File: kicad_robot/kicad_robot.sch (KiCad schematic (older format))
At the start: 1 part

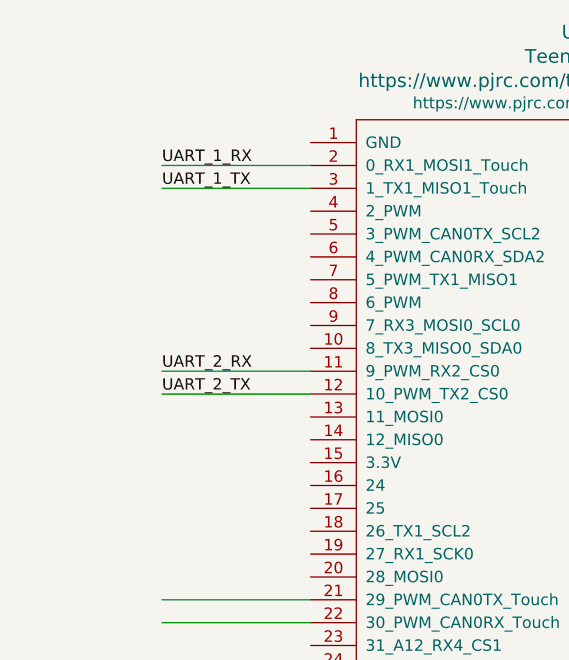
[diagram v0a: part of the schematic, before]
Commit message: Avancement sur la carte
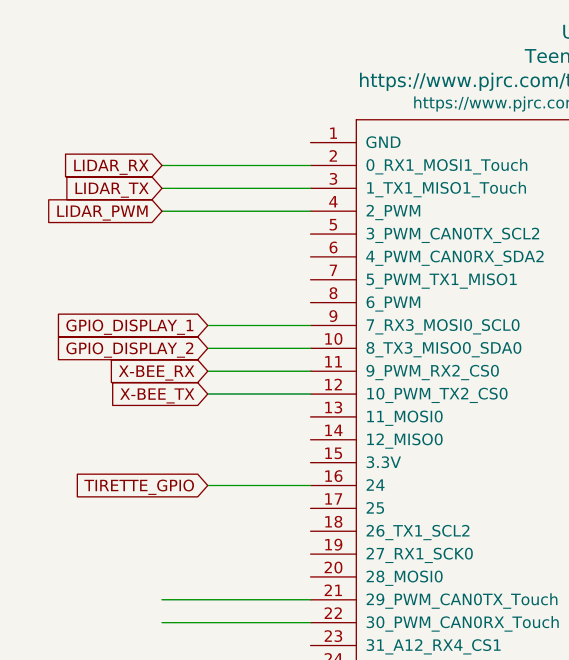
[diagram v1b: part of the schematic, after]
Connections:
- net labels added: GPIO_DISPLAY_1, GPIO_DISPLAY_2, LIDAR_PWM, LIDAR_RX, LIDAR_TX, TIRETTE_GPIO, X-BEE_RX, X-BEE_TX
- net labels removed: UART_1_RX, UART_1_TX, UART_2_RX, UART_2_TX
- wire segments 6 -> 10
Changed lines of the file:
@@
 Wire Wire Line
 	4550 2050 3900 2050
-Text Label 3900 1950 0    50   ~ 0
-UART_1_RX
-Text Label 3900 2050 0    50   ~ 0
-UART_1_TX
-Wire Wire Line
-	4550 2850 3900 2850
-Wire Wire Line
-	4550 2950 3900 2950
-Text Label 3900 2850 0    50   ~ 0
-UART_2_RX
-Text Label 3900 2950 0    50   ~ 0
-UART_2_TX
 Wire Wire Line
 	4550 3850 3900 3850
 Wire Wire Line
 	4550 3950 3900 3950
+Text GLabel 3900 1950 0    50   Input ~ 0
+LIDAR_RX
+Text GLabel 3900 2050 0    50   Input ~ 0
+LIDAR_TX
+Text GLabel 3900 2150 0    50   Input ~ 0
+LIDAR_PWM
+Wire Wire Line
+	3900 2150 4550 2150
+Text GLabel 4100 2650 0    50   Input ~ 0
+GPIO_DISPLAY_1
+Text GLabel 4100 2750 0    50   Input ~ 0
+GPIO_DISPLAY_2
+Wire Wire Line
+	4100 2750 4550 2750
+Wire Wire Line
+	4550 2650 4100 2650
+Text GLabel 4100 2850 0    50   Input ~ 0
+X-BEE_RX
+Text GLabel 4100 2950 0    50   Input ~ 0
+X-BEE_TX
+Wire Wire Line
+	4100 2950 4550 2950
+Wire Wire Line
+	4100 2850 4550 2850
+Text GLabel 4100 3350 0    50   Input ~ 0
+TIRETTE_GPIO
+Wire Wire Line
+	4100 3350 4550 3350
 $EndSCHEMATC

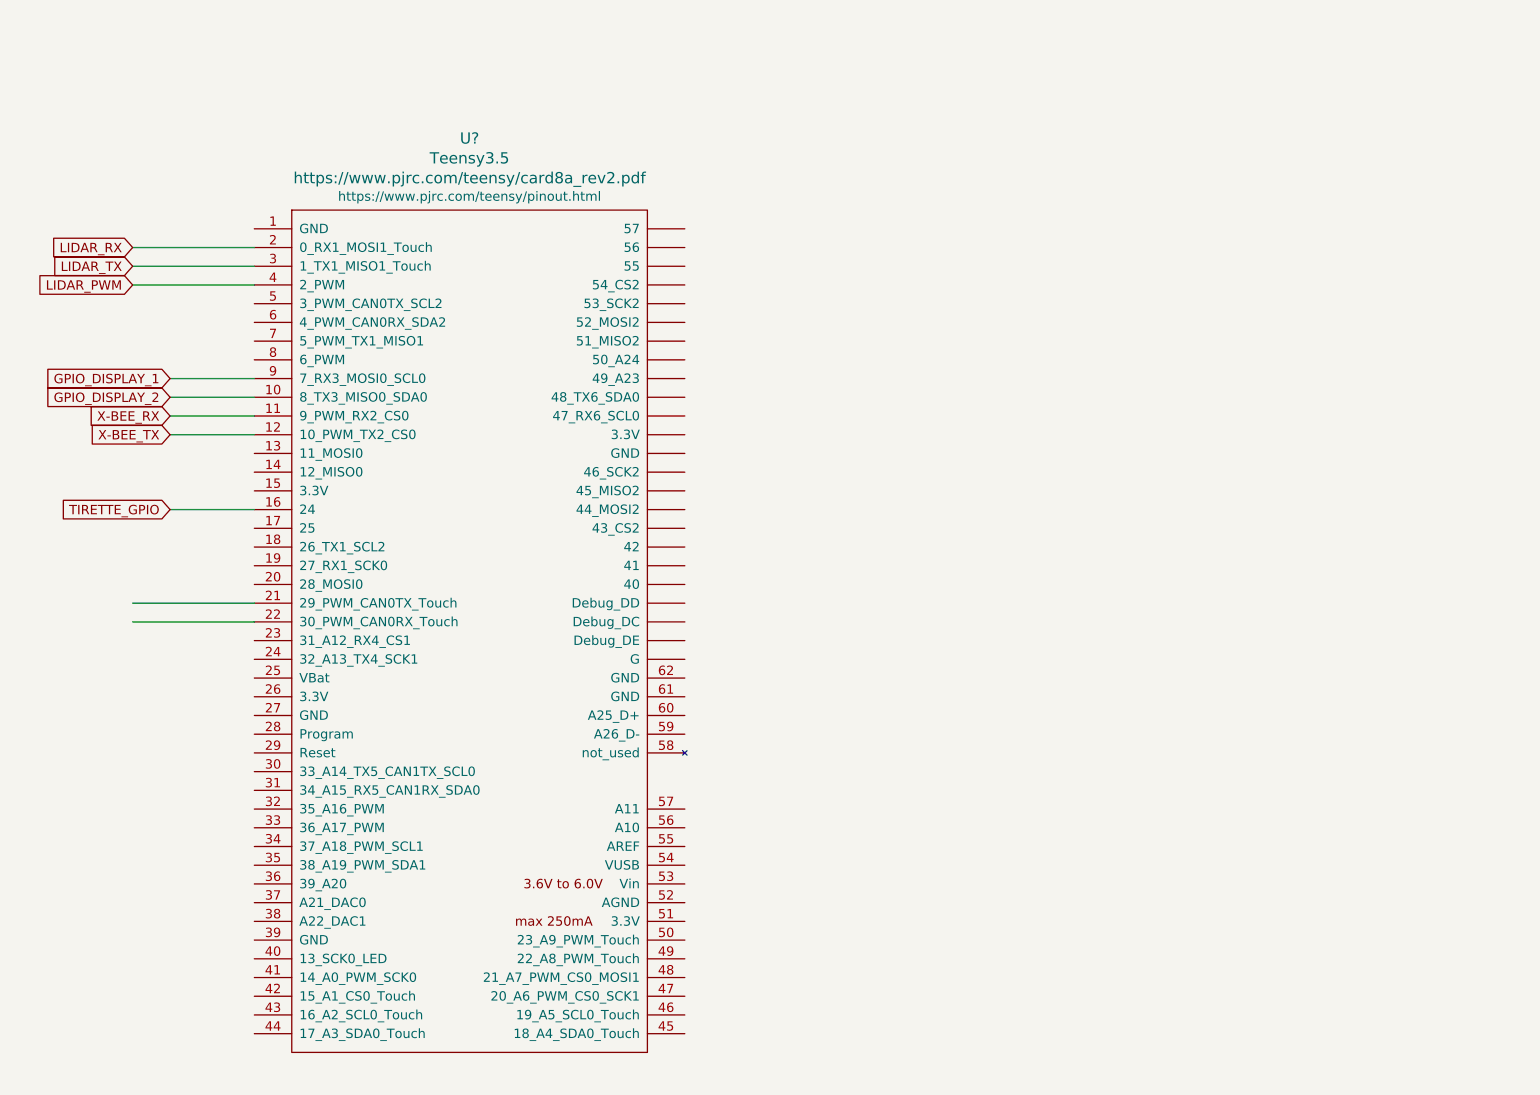
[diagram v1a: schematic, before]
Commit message: Petit avancement
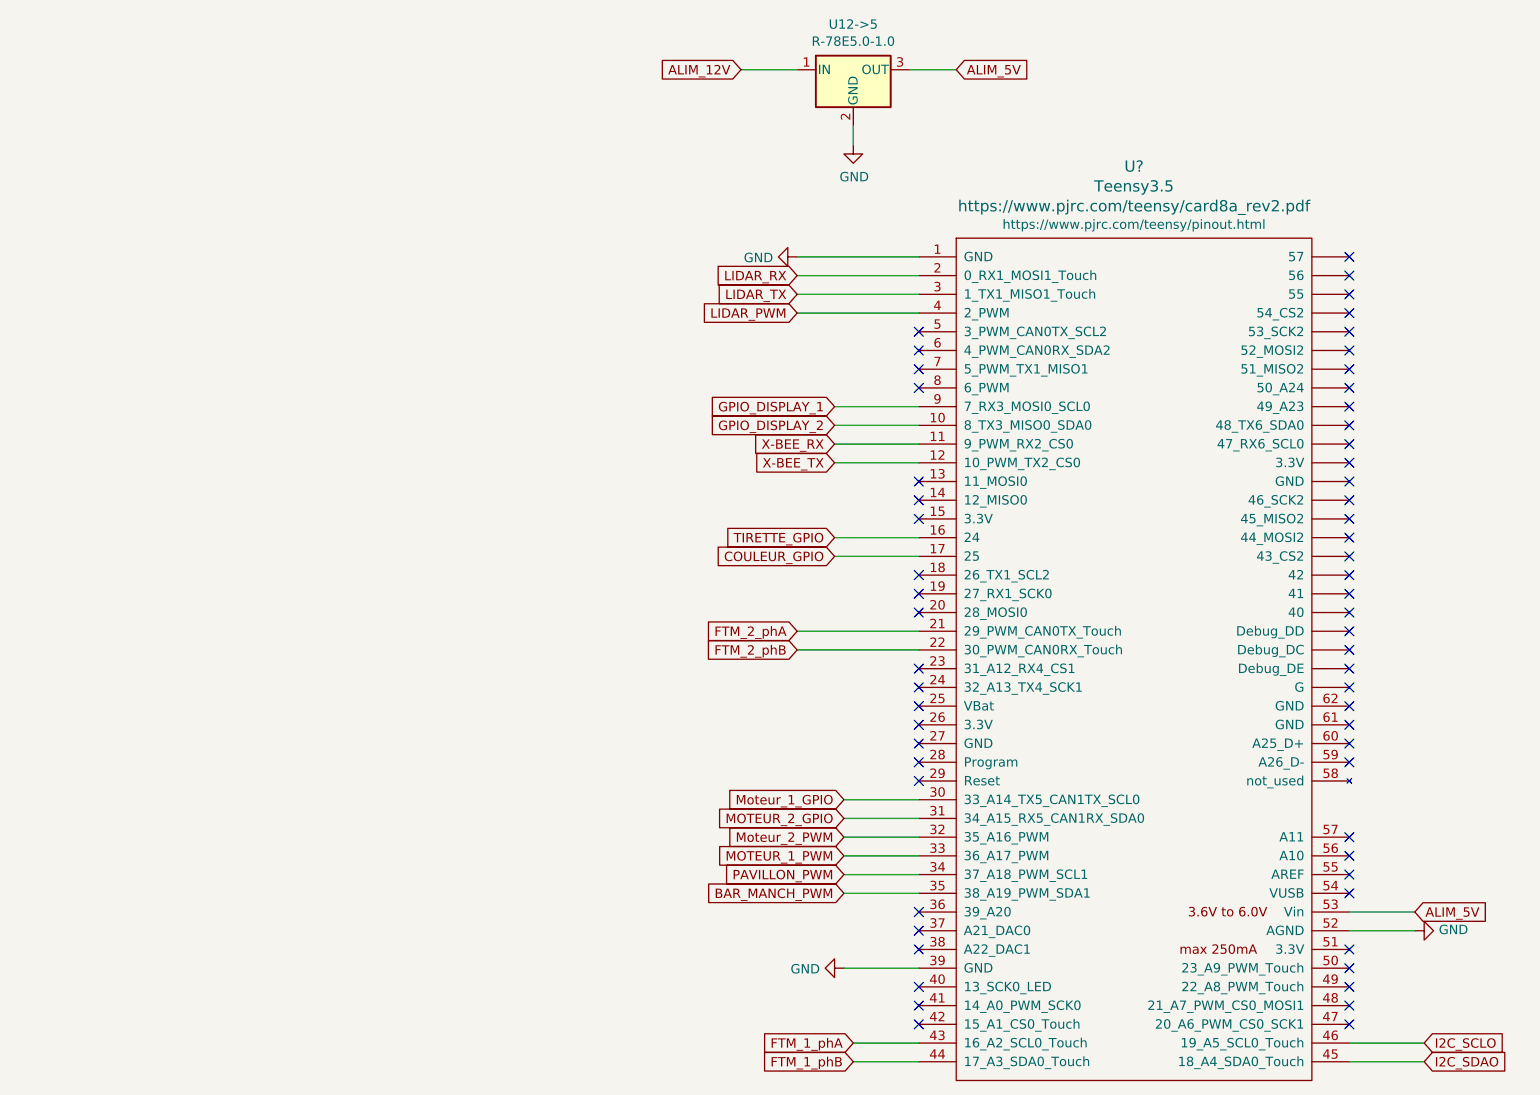
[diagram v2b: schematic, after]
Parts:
- added U12->5: R-78E5.0-1.0, Converter_DCDC:Converter_DCDC_RECOM_R-78E-0.5_THT, symbol Regulator_Switching:R-78E5.0-1.0
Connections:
- net labels added: ALIM_12V, ALIM_5V, BAR_MANCH_PWM, COULEUR_GPIO, FTM_1_phA, FTM_1_phB, FTM_2_phA, FTM_2_phB, GND, I2C_SCLO, I2C_SDAO, MOTEUR_1_PWM, MOTEUR_2_GPIO, Moteur_1_GPIO, Moteur_2_PWM, PAVILLON_PWM
- wire segments 10 -> 28
- no-connect marks 0 -> 60
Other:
- moved on the sheet: U?
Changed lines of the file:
@@
 L teensy:Teensy3.5 U?
 U 1 1 6026B470
-P 5700 4000
-F 0 "U?" H 5700 6633 60  0000 C CNN
-F 1 "Teensy3.5" H 5700 6527 60  0000 C CNN
-F 2 "" H 5600 6250 60  0000 C CNN
-F 3 "https://www.pjrc.com/teensy/card8a_rev2.pdf" H 5700 6421 60  0000 C CNN
-F 4 "https://www.pjrc.com/teensy/pinout.html" H 5700 6323 50  0000 C CNN "Pinouts"
-	1    5700 4000
+P 9250 4150
+F 0 "U?" H 9250 6783 60  0000 C CNN
+F 1 "Teensy3.5" H 9250 6677 60  0000 C CNN
+F 2 "" H 9150 6400 60  0000 C CNN
+F 3 "https://www.pjrc.com/teensy/card8a_rev2.pdf" H 9250 6571 60  0000 C CNN
+F 4 "https://www.pjrc.com/teensy/pinout.html" H 9250 6473 50  0000 C CNN "Pinouts"
+	1    9250 4150
 	1    0    0    -1
 $EndComp
-Wire Wire Line
-	4550 1950 3900 1950
-Wire Wire Line
-	4550 2050 3900 2050
-Wire Wire Line
-	4550 3850 3900 3850
-Wire Wire Line
-	4550 3950 3900 3950
-Text GLabel 3900 1950 0    50   Input ~ 0
+Text GLabel 7450 2100 0    50   Input ~ 0
 LIDAR_RX
-Text GLabel 3900 2050 0    50   Input ~ 0
+Text GLabel 7450 2200 0    50   Input ~ 0
 LIDAR_TX
-Text GLabel 3900 2150 0    50   Input ~ 0
+Text GLabel 7450 2300 0    50   Input ~ 0
 LIDAR_PWM
-Wire Wire Line
-	3900 2150 4550 2150
-Text GLabel 4100 2650 0    50   Input ~ 0
+Text GLabel 7650 2800 0    50   Input ~ 0
 GPIO_DISPLAY_1
-Text GLabel 4100 2750 0    50   Input ~ 0
+Text GLabel 7650 2900 0    50   Input ~ 0
 GPIO_DISPLAY_2
-Wire Wire Line
-	4100 2750 4550 2750
-Wire Wire Line
-	4550 2650 4100 2650
-Text GLabel 4100 2850 0    50   Input ~ 0
+Text GLabel 7650 3000 0    50   Input ~ 0
 X-BEE_RX
-Text GLabel 4100 2950 0    50   Input ~ 0
+Text GLabel 7650 3100 0    50   Input ~ 0
 X-BEE_TX
-Wire Wire Line
-	4100 2950 4550 2950
-Wire Wire Line
-	4100 2850 4550 2850
-Text GLabel 4100 3350 0    50   Input ~ 0
+Text GLabel 7650 3500 0    50   Input ~ 0
 TIRETTE_GPIO
-Wire Wire Line
-	4100 3350 4550 3350
+$Comp
+L power:GND #PWR?
+U 1 1 60316113
+P 7450 2000
+F 0 "#PWR?" H 7450 1750 50  0001 C CNN
+F 1 "GND" V 7455 1872 50  0000 R CNN
+F 2 "" H 7450 2000 50  0001 C CNN
+F 3 "" H 7450 2000 50  0001 C CNN
+	1    7450 2000
+	0    1    1    0
+$EndComp
+Text GLabel 10750 5500 2    50   Input ~ 0
+ALIM_5V
+Wire Wire Line
+	10750 5500 10400 5500
+Text GLabel 7650 3600 0    50   Input ~ 0
+COULEUR_GPIO
+Text GLabel 7450 4000 0    50   Input ~ 0
+FTM_2_phA
+Text GLabel 7450 4100 0    50   Input ~ 0
+FTM_2_phB
+Text GLabel 7700 4900 0    50   Input ~ 0
+Moteur_1_GPIO
+Text GLabel 7700 5000 0    50   Input ~ 0
+MOTEUR_2_GPIO
+Text GLabel 7700 5100 0    50   Input ~ 0
+Moteur_2_PWM
+Text GLabel 7700 5200 0    50   Input ~ 0
+MOTEUR_1_PWM
+Text GLabel 7700 5300 0    50   Input ~ 0
+PAVILLON_PWM
+Text GLabel 7700 5400 0    50   Input ~ 0
+BAR_MANCH_PWM
+Text GLabel 7750 6200 0    50   Input ~ 0
+FTM_1_phA
+Text GLabel 7750 6300 0    50   Input ~ 0
+FTM_1_phB
+Wire Wire Line
+	7750 6300 8100 6300
+Text GLabel 10800 6300 2    50   Input ~ 0
+I2C_SDAO
+Text GLabel 10800 6200 2    50   Input ~ 0
+I2C_SCLO
+Wire Wire Line
+	10400 6300 10800 6300
+Wire Wire Line
+	10800 6200 10400 6200
+$Comp
+L power:GND #PWR?
+U 1 1 6033D90A
+P 10750 5600
+F 0 "#PWR?" H 10750 5350 50  0001 C CNN
+F 1 "GND" V 10755 5472 50  0000 R CNN
+F 2 "" H 10750 5600 50  0001 C CNN
+F 3 "" H 10750 5600 50  0001 C CNN
+	1    10750 5600
+	0    -1   -1   0
+$EndComp
+Wire Wire Line
+	10750 5600 10400 5600
+NoConn ~ 10400 4300
+NoConn ~ 10400 4200
+NoConn ~ 10400 4100
+NoConn ~ 10400 4000
+Wire Wire Line
+	7450 2100 8100 2100
+Wire Wire Line
+	7450 2200 8100 2200
+Wire Wire Line
+	7450 4000 8100 4000
+Wire Wire Line
+	7450 4100 8100 4100
+Wire Wire Line
+	7450 2300 8100 2300
+Wire Wire Line
+	7650 2900 8100 2900
+Wire Wire Line
+	7650 2800 8100 2800
+Wire Wire Line
+	7650 3100 8100 3100
+Wire Wire Line
+	7650 3000 8100 3000
+Wire Wire Line
+	7650 3500 8100 3500
+Wire Wire Line
+	7450 2000 8100 2000
+Wire Wire Line
+	7650 3600 8100 3600
+Wire Wire Line
+	7700 5400 8100 5400
+Wire Wire Line
+	7700 5300 8100 5300
+Wire Wire Line
+	7700 5200 8100 5200
+Wire Wire Line
+	7700 5100 8100 5100
+Wire Wire Line
+	7700 5000 8100 5000
+Wire Wire Line
+	7700 4900 8100 4900
+Wire Wire Line
+	7750 6200 8100 6200
+NoConn ~ 10400 3900
+NoConn ~ 10400 3800
+NoConn ~ 10400 3700
+NoConn ~ 10400 3600
+NoConn ~ 10400 3500
+NoConn ~ 10400 3400
+NoConn ~ 10400 3300
+NoConn ~ 10400 3200
+NoConn ~ 10400 3100
+NoConn ~ 10400 3000
+NoConn ~ 10400 2900
+NoConn ~ 10400 2800
+NoConn ~ 10400 2700
+NoConn ~ 10400 2600
+NoConn ~ 10400 2500
+NoConn ~ 10400 2400
+NoConn ~ 10400 2300
+NoConn ~ 10400 2000
+NoConn ~ 10400 2100
+NoConn ~ 10400 2200
+NoConn ~ 8100 2400
+NoConn ~ 8100 2500
+NoConn ~ 8100 2600
+NoConn ~ 8100 2700
+NoConn ~ 8100 3200
+NoConn ~ 8100 3300
+NoConn ~ 8100 3400
+NoConn ~ 8100 3700
+NoConn ~ 8100 3800
+NoConn ~ 8100 3900
+NoConn ~ 8100 4200
+NoConn ~ 8100 4300
+NoConn ~ 8100 4400
+NoConn ~ 8100 4500
+NoConn ~ 8100 4600
+NoConn ~ 8100 4700
+NoConn ~ 8100 4800
+NoConn ~ 8100 5500
+NoConn ~ 8100 5600
+NoConn ~ 8100 5700
+NoConn ~ 8100 5900
+NoConn ~ 8100 6000
+NoConn ~ 8100 6100
+NoConn ~ 10400 6100
+NoConn ~ 10400 6000
+NoConn ~ 10400 5900
+NoConn ~ 10400 5800
+NoConn ~ 10400 5700
+NoConn ~ 10400 5400
+NoConn ~ 10400 5300
+NoConn ~ 10400 5200
+NoConn ~ 10400 5100
+NoConn ~ 10400 4700
+NoConn ~ 10400 4600
+NoConn ~ 10400 4500
+NoConn ~ 10400 4400
+$Comp
+L power:GND #PWR?
+U 1 1 6036B9DC
+P 7700 5800
+F 0 "#PWR?" H 7700 5550 50  0001 C CNN
+F 1 "GND" V 7705 5672 50  0000 R CNN
+F 2 "" H 7700 5800 50  0001 C CNN
+F 3 "" H 7700 5800 50  0001 C CNN
+	1    7700 5800
+	0    1    1    0
+$EndComp
+Wire Wire Line
+	7700 5800 8100 5800
+$Comp
+L Regulator_Switching:R-78E5.0-1.0 U12->5
+U 1 1 6037B063
+P 7750 1000
+F 0 "U12->5" H 7750 1242 50  0000 C CNN
+F 1 "R-78E5.0-1.0" H 7750 1151 50  0000 C CNN
+F 2 "Converter_DCDC:Converter_DCDC_RECOM_R-78E-0.5_THT" H 7800 750 50  0001 L CIN
+F 3 "https://www.recom-power.com/pdf/Innoline/R-78Exx-1.0.pdf" H 7750 1000 50  0001 C CNN
+	1    7750 1000
+	1    0    0    -1
+$EndComp
+Text GLabel 8300 1000 2    50   Input ~ 0
+ALIM_5V
+Wire Wire Line
+	8300 1000 8050 1000
+$Comp
+L power:GND #PWR?
+U 1 1 6037D422
+P 7750 1400
+F 0 "#PWR?" H 7750 1150 50  0001 C CNN
+F 1 "GND" H 7755 1227 50  0000 C CNN
+F 2 "" H 7750 1400 50  0001 C CNN
+F 3 "" H 7750 1400 50  0001 C CNN
+	1    7750 1400
+	1    0    0    -1
+$EndComp
+Wire Wire Line
+	7750 1400 7750 1300
+Text GLabel 7150 1000 0    50   Input ~ 0
+ALIM_12V
+Wire Wire Line
+	7150 1000 7450 1000
 $EndSCHEMATC
